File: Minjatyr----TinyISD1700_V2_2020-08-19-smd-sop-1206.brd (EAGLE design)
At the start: 40.5 x 49.2 mm, 20 parts, among them IC3 LM317MDT, J1 AVR_SPI_PRG_6OFFSET_PADS, U1 ATTINY4313-SU

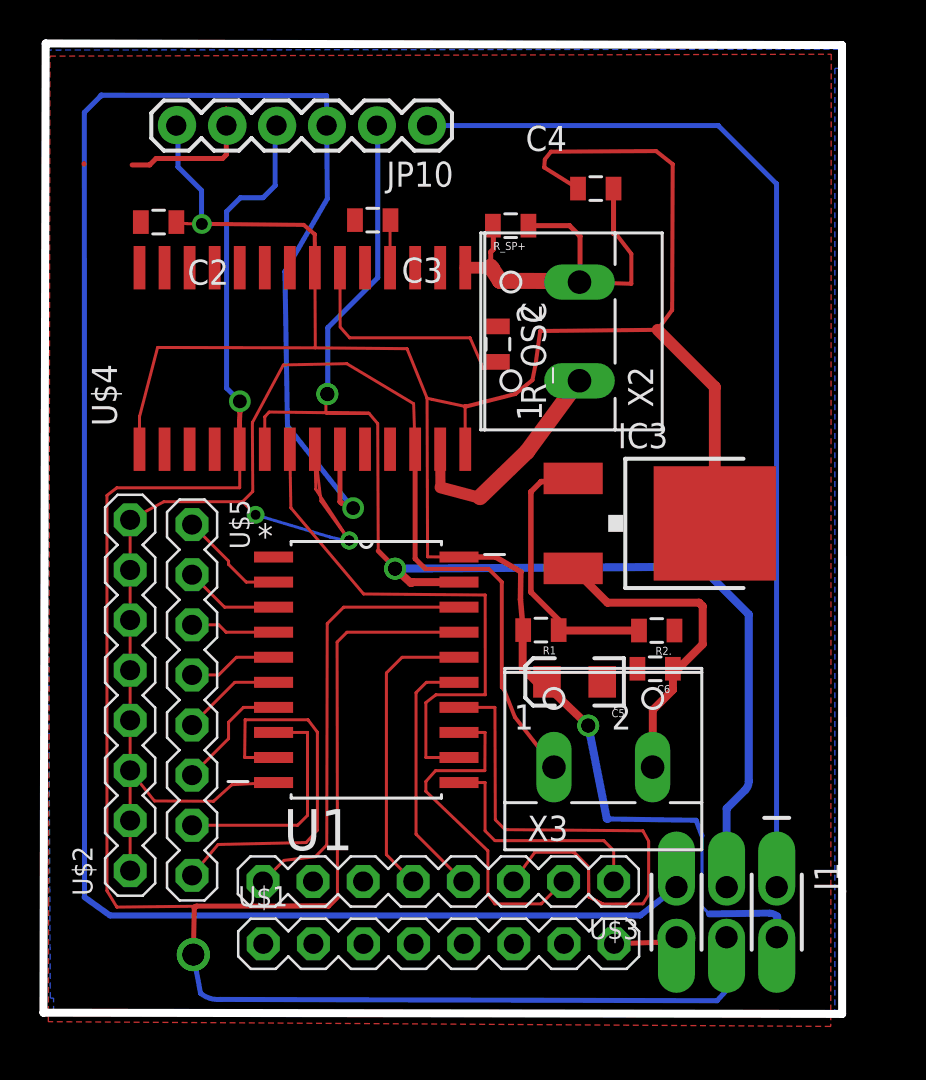
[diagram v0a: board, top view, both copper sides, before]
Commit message: commit
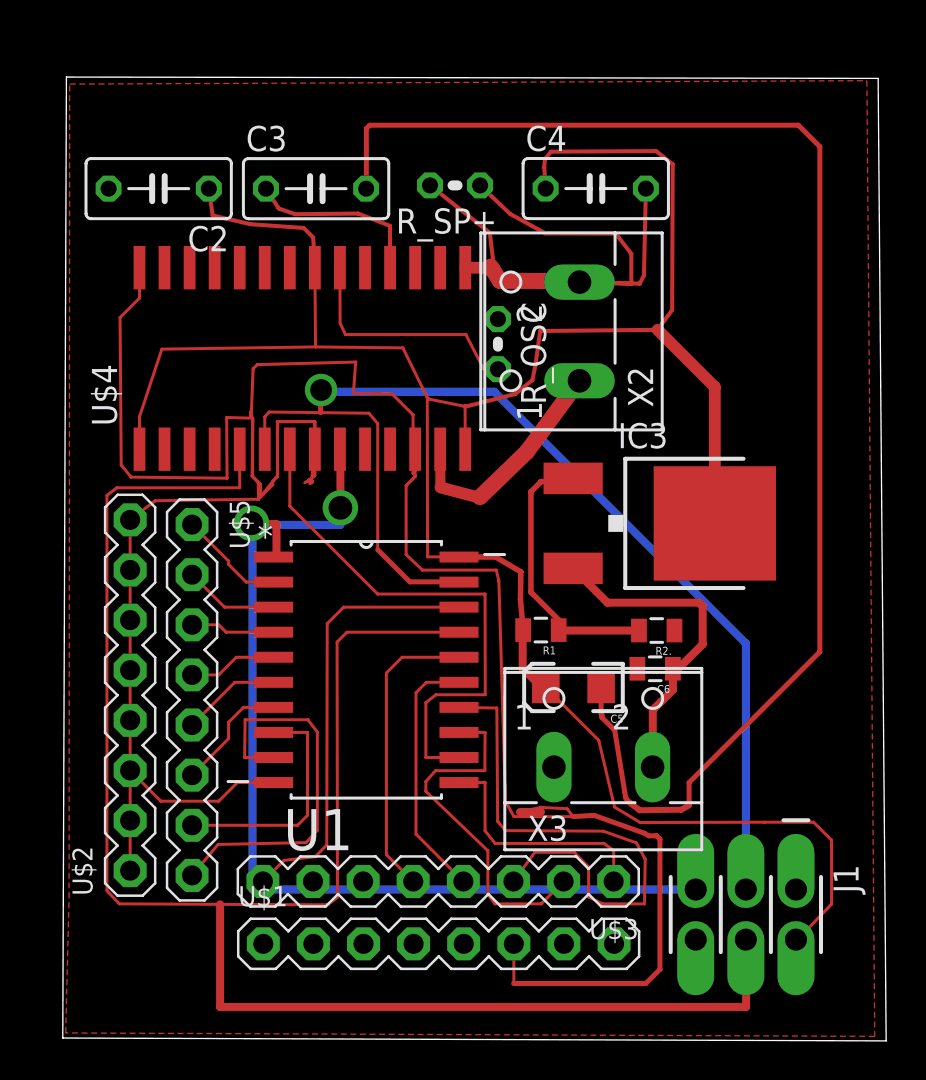
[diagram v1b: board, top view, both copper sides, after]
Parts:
- removed JP10: (no value), SparkFun-Connectors:1X06
- C2, C3, C4: device SparkFun2:0805 -> resistor:C050-030X075
- R_OSC, R_SP+: device SparkFun2:0805 -> rcl:0204V
- moved R_SP+ 3.48 mm to (17.8, 39.6)
- moved C3 3.28 mm to (10.7, 39.5), turned to 0 degrees
- moved C2 1.70 mm to (2.75, 39.5)
- moved J1 0.98 mm to (32.5, 2.68)
- moved C5 0.29 mm to (23.8, 14.2)
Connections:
- net ANALN: now also U1.1; no longer JP10.3
- net CSK: no longer JP10.2
- net GND: no longer JP10.5
- net MISO: no longer JP10.1
- net MOSI: no longer JP10.4
- net VCC: no longer JP10.6
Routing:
- net GND: track 100.9 -> 221.6 mm, vias 3 -> 0
- net ANALN: track 112.7 -> 52.3 mm, vias 1 -> 0
- net MISO: track 54.6 -> 0.00 mm
- net MOSI: track 120.5 -> 95.6 mm, vias 2 -> 0
- net CSK: track 73.5 -> 59.4 mm, vias 2 -> 0
- net N$4: track 13.0 -> 21.1 mm
- net N$5: track 2.42 -> 9.12 mm
- net VCC: track 126.6 -> 121.2 mm, vias 2 -> 0
- net N$3: track 31.6 -> 27.5 mm
- net N$7: track 8.75 -> 12.3 mm
- removed copper zone on layer 16, net GND
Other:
- board size 40.5 x 49.2 mm -> 41.7 x 48.9 mm
